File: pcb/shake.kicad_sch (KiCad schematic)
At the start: 13 parts, among them U1 MSP430G2553, U2 BST, U3 SW-420

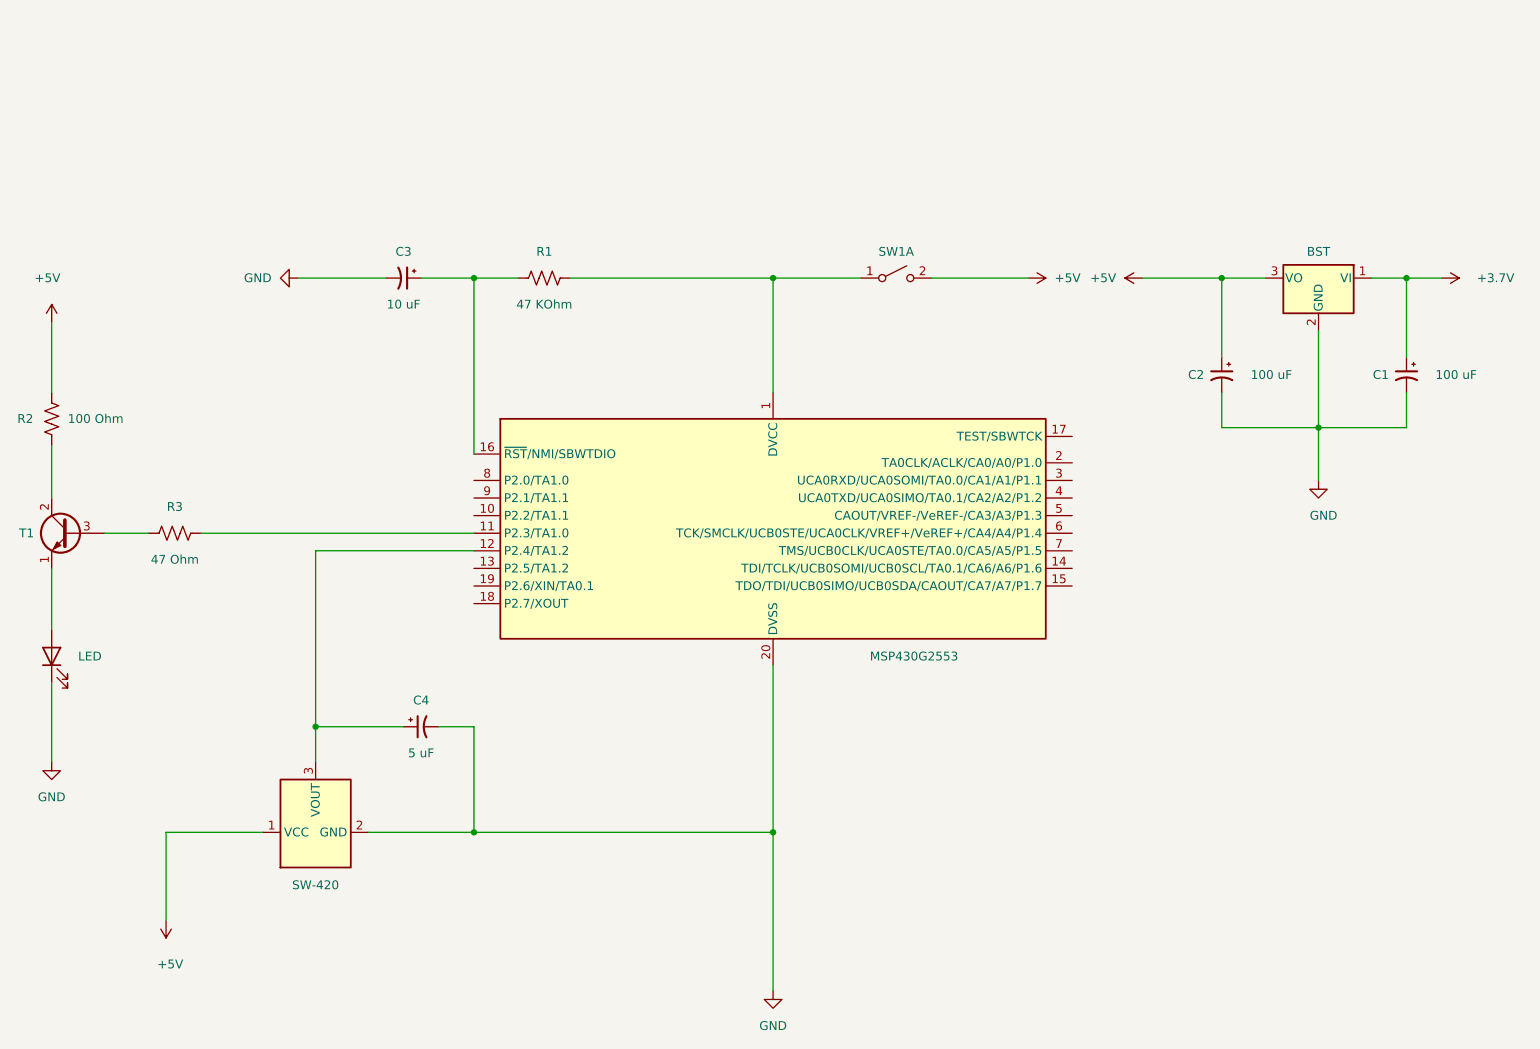
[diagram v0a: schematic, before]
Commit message: Update pcb and schematics
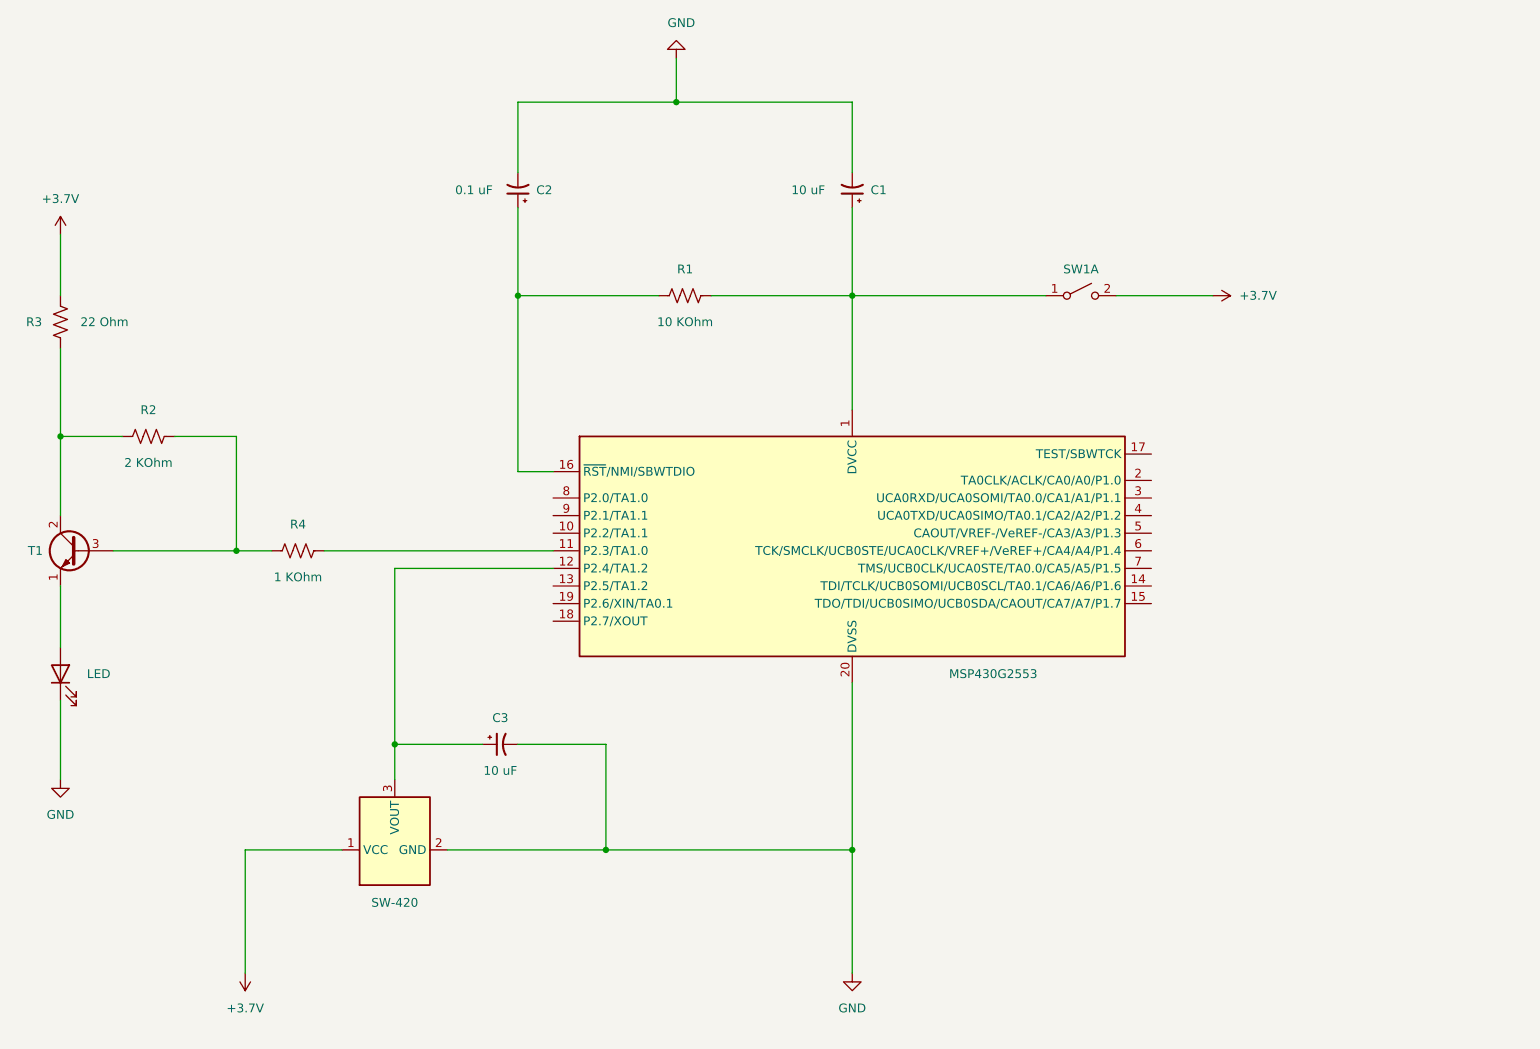
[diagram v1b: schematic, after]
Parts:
- removed C2: 100 uF, symbol Device:C_Polarized_Small_US
- removed U2: BST, Package_TO_SOT_THT:TO-220-3_Vertical, symbol Regulator_Linear:SPX2920U-5.0_TO220
- added R2: 2 KOhm, symbol Device:R_US
- C1: value 100 uF -> 10 uF
- C2: renamed from C3; value 10 uF -> 0.1 uF
- C3: renamed from C4; value 5 uF -> 10 uF
- R1: value 47 KOhm -> 10 KOhm
- R3: renamed from R2; value 100 Ohm -> 22 Ohm
- R4: renamed from R3; value 47 Ohm -> 1 KOhm
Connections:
- net +3.7V is gone; now on an unnamed net: C1.1
- net at R3.1, T1.2 (C): now also R2.1
- net at R4.2, T1.3 (B): now also R2.2
- net +5V renamed +3.3VDAC
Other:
- company: (none) -> Maksym Dybarskyi
- title: (none) -> Shake LED
- moved on the sheet: C2, C3, R1, R3, R4, SW1A, T1
